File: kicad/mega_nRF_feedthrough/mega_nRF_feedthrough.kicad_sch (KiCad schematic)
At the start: 13 parts, among them J1 Conn_01x08_Pin, J2 Conn_01x08_Pin, J3 Conn_01x10_Pin, J4 Conn_01x08_Pin, J6 Conn_01x08_Pin, J7 Conn_01x36, J8 Conn_01x06, U1 NRF24L01_Breakout, U2 AP2127N-3.3

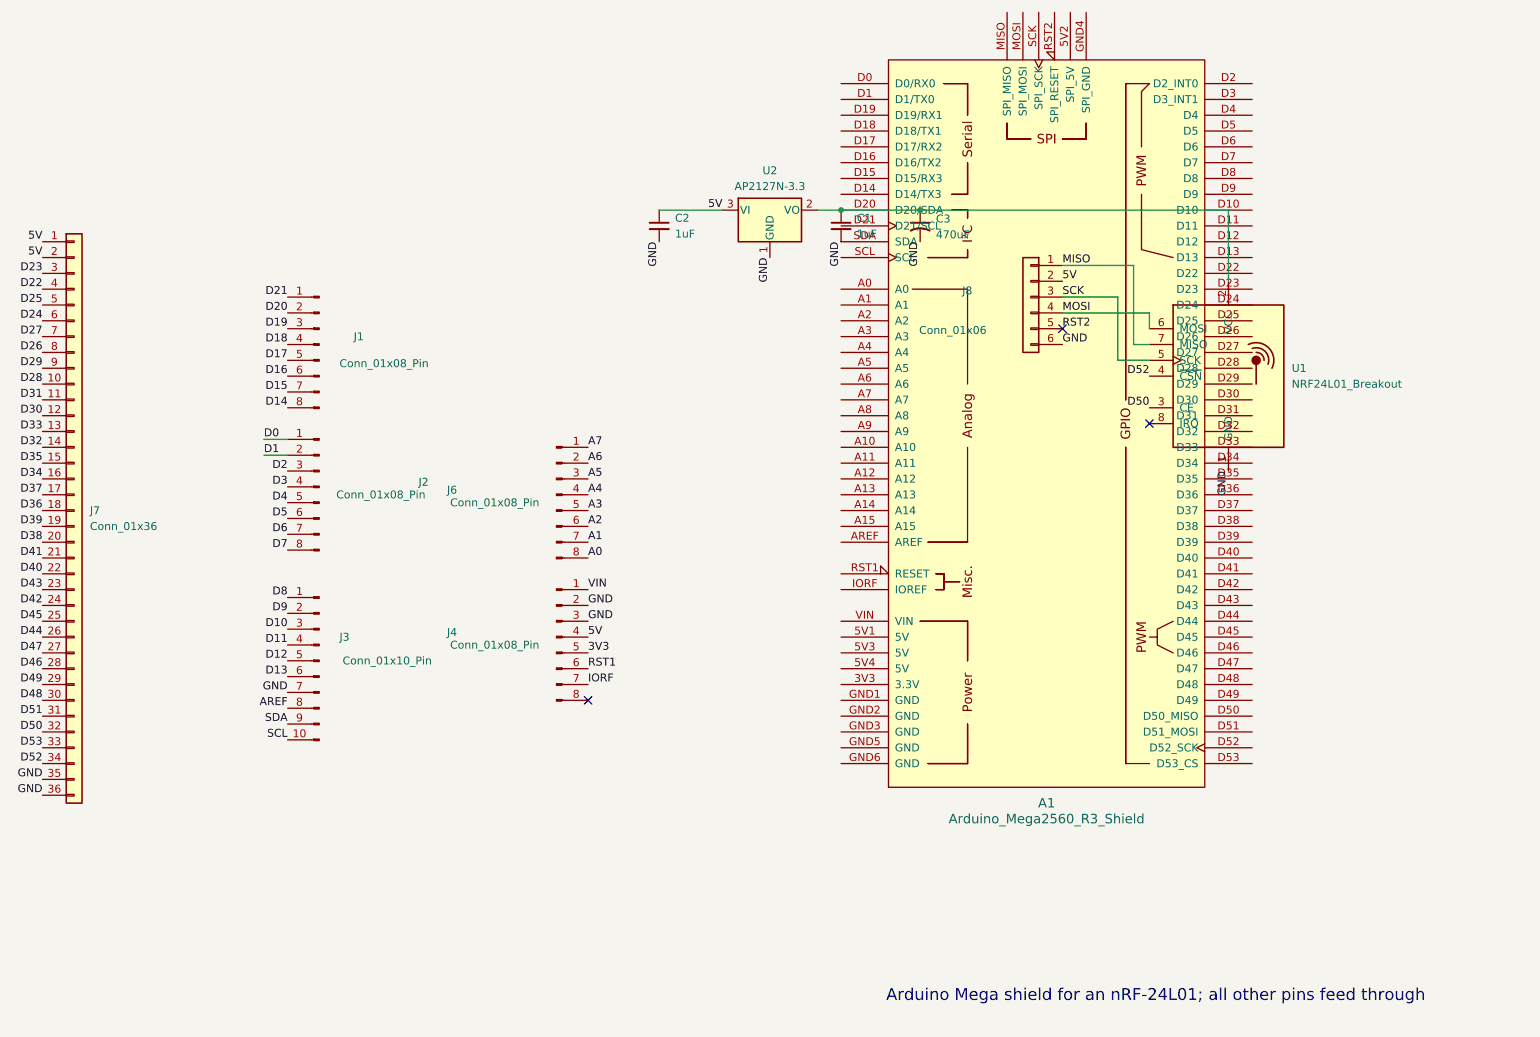
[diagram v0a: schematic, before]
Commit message: done
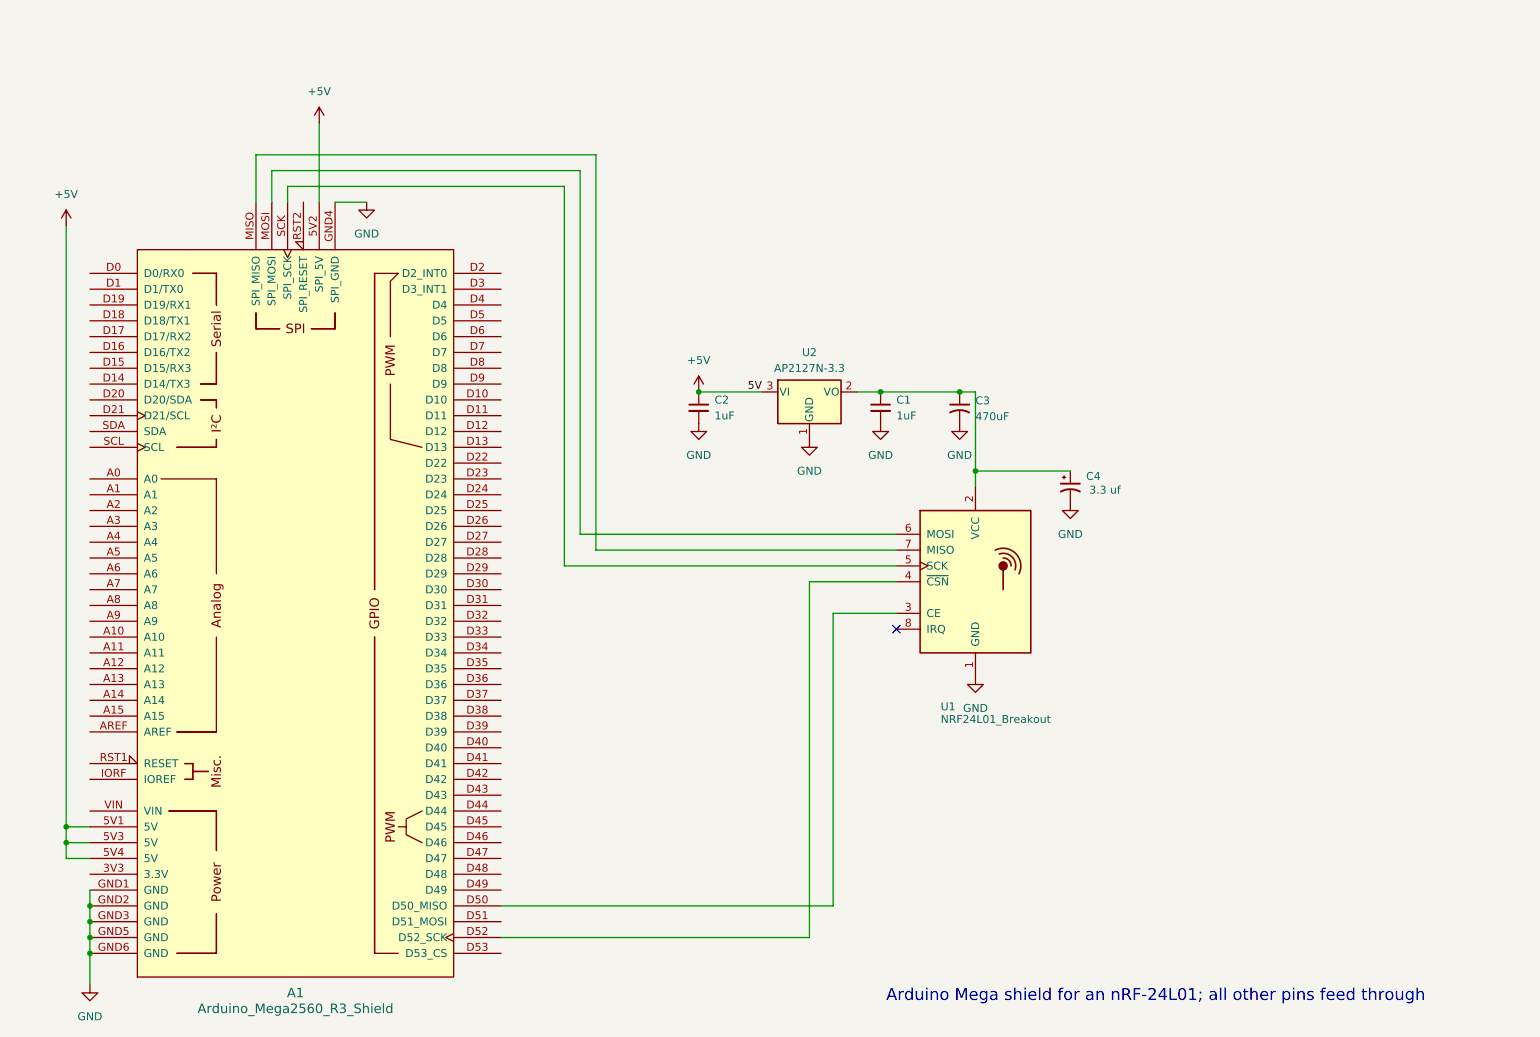
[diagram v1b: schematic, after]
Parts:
- removed J1, J2, J4, J6: Conn_01x08_Pin, Connector_PinHeader_2.54mm:PinHeader_1x08_P2.54mm_Vertical, symbol Connector:Conn_01x08_Pin
- removed J3: Conn_01x10_Pin, Connector_PinHeader_2.54mm:PinHeader_1x10_P2.54mm_Vertical, symbol Connector:Conn_01x10_Pin
- removed J7: Conn_01x36, Connector_PinHeader_2.54mm:PinHeader_2x18_P2.54mm_Vertical, symbol Connector_Generic:Conn_01x36
- removed J8: Conn_01x06, Connector_PinHeader_2.54mm:PinHeader_2x03_P2.54mm_Vertical, symbol Connector_Generic:Conn_01x06
- added C4: 3.3 uf, Capacitor_Tantalum_SMD:CP_EIA-3216-18_Kemet-A, symbol Device:C_Polarized_Small_US
- C3: footprint (none) -> Capacitor_THT:CP_Radial_D8.0mm_P3.50mm
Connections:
- net 5V is gone; now on net +5V: C2.1, U2.3 (VI)
- net D50 is gone; now on an unnamed net: U1.3 (CE)
- net D52 is gone; now on an unnamed net: U1.4 (~{CSN})
- net MISO is gone; now on an unnamed net: U1.7 (MISO)
- net MOSI is gone; now on an unnamed net: U1.6 (MOSI)
- net SCK is gone; now on an unnamed net: U1.5 (SCK)
- net GND: now also A1.GND1 (GND), A1.GND2 (GND), A1.GND3 (GND), A1.GND4 (SPI_GND), A1.GND5 (GND), A1.GND6 (GND), C4.2; no longer A1.SDA
- net at C1.1, C3.1, U1.2 (VCC)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: now also C4.1; no longer A1.D20 (D20/SDA)
- net +5V: now reaches A1.5V1 (5V)
- net +5V: now also A1.5V2 (SPI_5V), A1.5V3 (5V), A1.5V4 (5V)
- no-connect marks 3 -> 1
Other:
- moved on the sheet: A1, C1, C2, C3, U1, U2
